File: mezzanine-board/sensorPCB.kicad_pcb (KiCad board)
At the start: 2 copper layers, 50 x 12.5 mm, 22 parts, among them J1 SFMC-105-01-L-D, U1 AS72651, U2 4MB Flash, U3 AS72652, U4 AS72653

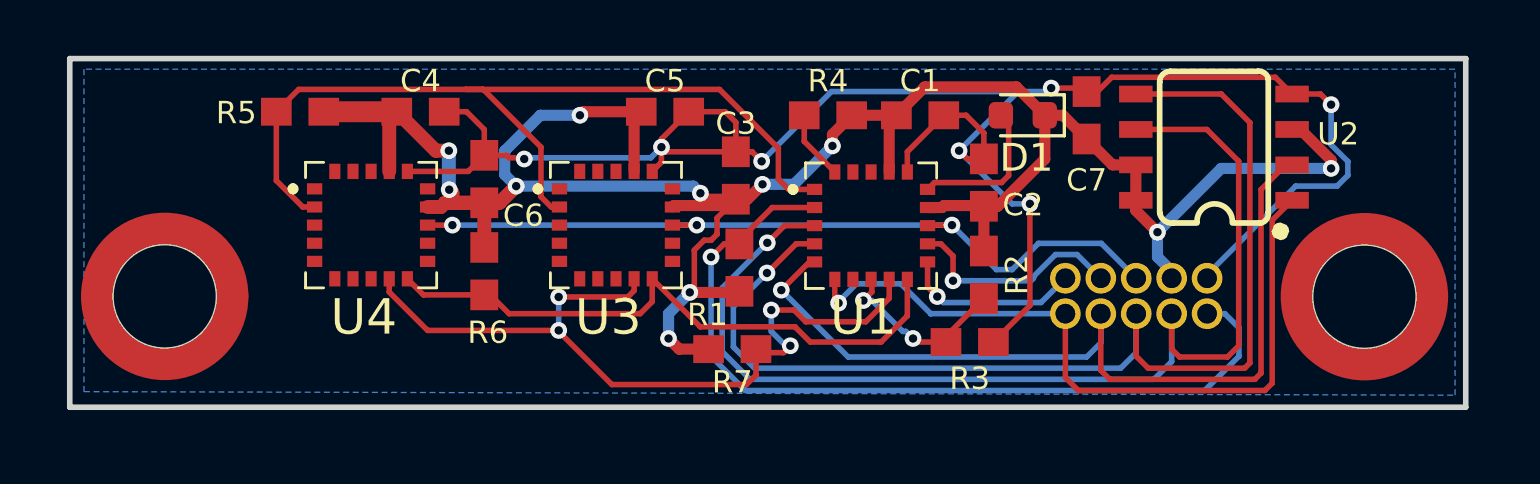
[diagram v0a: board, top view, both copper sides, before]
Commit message: Update larger board design
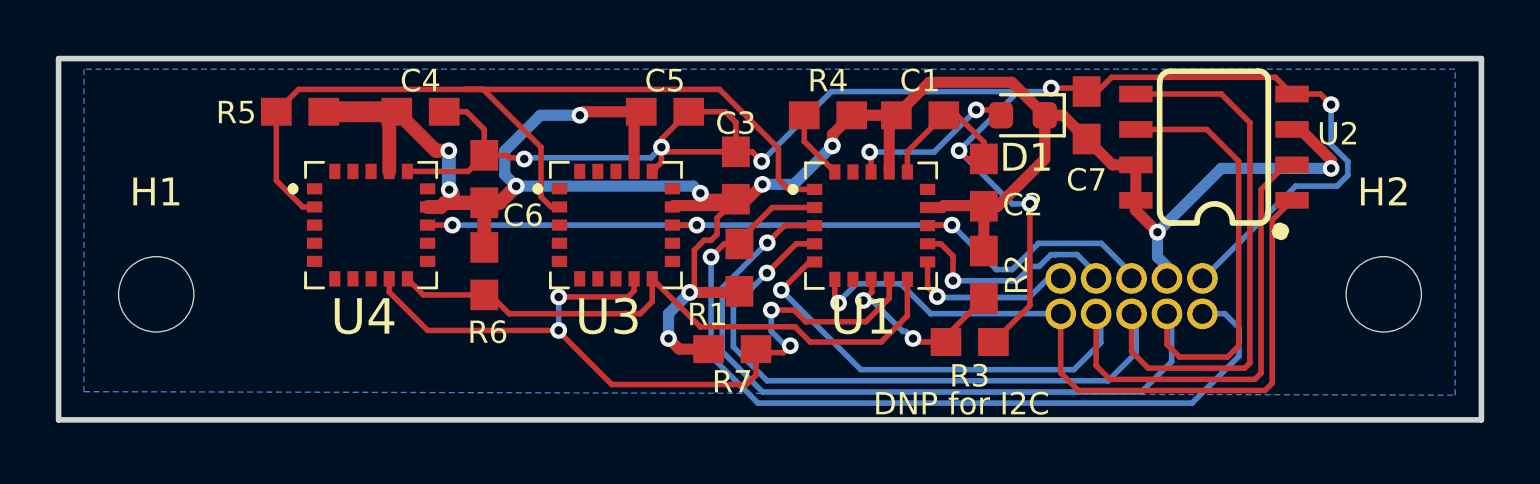
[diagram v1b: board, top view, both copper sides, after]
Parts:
- H1, H2: footprint Mounting_Wuerth:Mounting_Wuerth_WA-SMSI-M2.5_H0.5mm_9774005151 -> MountingHole:MountingHole_2.7mm_M2.5
- moved H2 0.70 mm to (136.0, 91.0)
- moved H1 0.31 mm to (92.0, 91.0)
- moved J1 0.17 mm to (124.4, 91.7)
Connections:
- U1 pad 15: Net-(D1-A) -> unconnected-(U1-LED_DRV-Pad15)
- U1 pad 18: unconnected-(U1-LED_IND-Pad18) -> Net-(D1-A)
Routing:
- net Net-(D1-A): track 5.39 -> 6.14 mm, vias 0 -> 2
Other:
- board size 50 x 12.5 mm -> 51 x 13 mm
- board text added: "DNP for I2C"
